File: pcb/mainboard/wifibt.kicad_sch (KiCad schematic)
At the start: 15 parts, among them U901 AP6330(BCM4330), Y901 26MHz

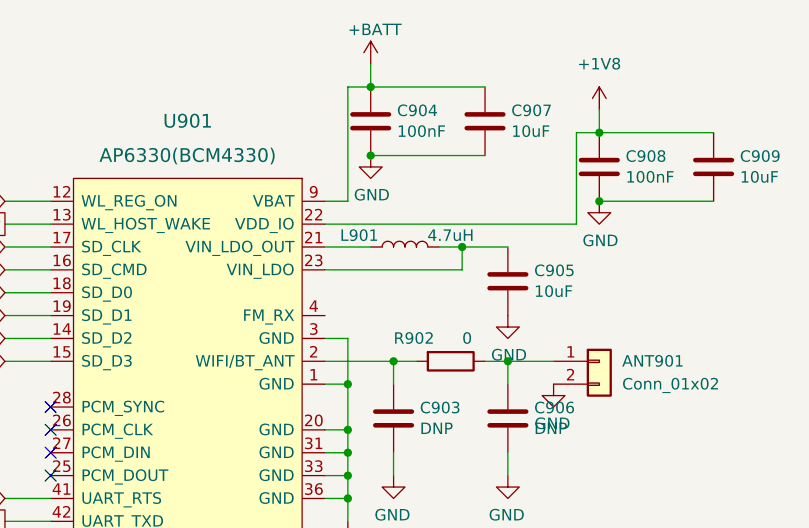
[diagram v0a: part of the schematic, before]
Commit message: Keypad bugfix, pulling in submodules
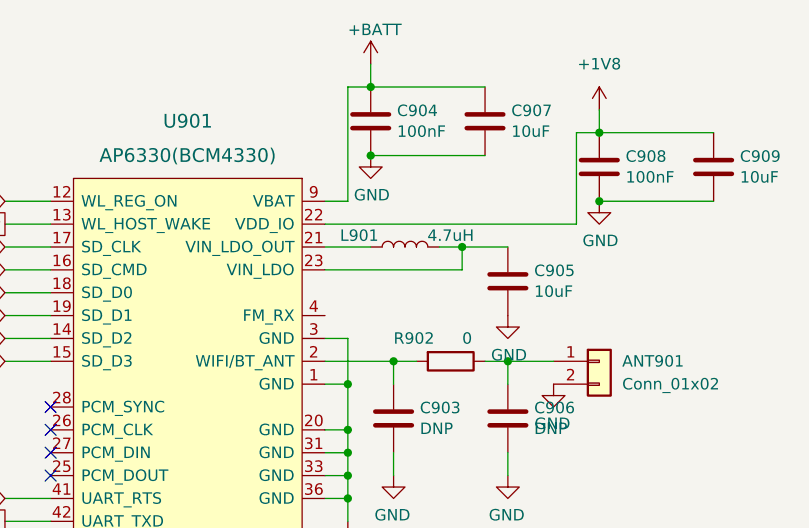
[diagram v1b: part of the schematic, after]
